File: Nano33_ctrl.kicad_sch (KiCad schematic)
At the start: 55 parts, among them J1 To Protec_Brd, J12 Conn_01x02, J15 To Display, J17 Conn_01x02, J18 To Protec_Brd encoder, J19 To P.A., J4 Power_In, J5 Conn_01x02, J6 Conn_01x02, U12 Arduino-NANO-33, U2 LM1117S-5.0, U3 LM1117S-3.3, U4 74HCT04, U5 TPIC6595, U6 TPIC6595, U7 TPIC6595, U8 24FC1025-I_SN, U9 24FC1025-I_SN

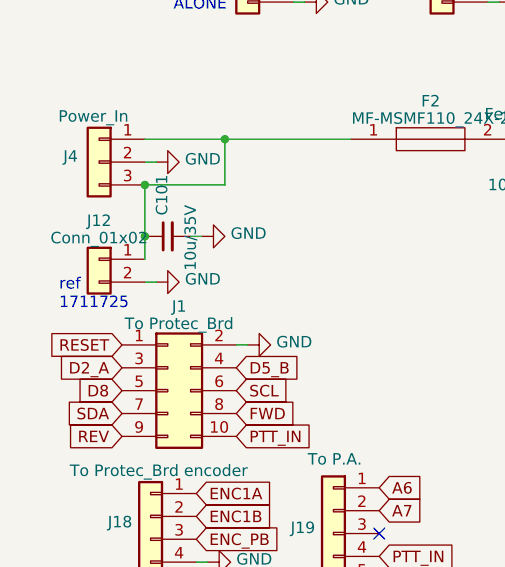
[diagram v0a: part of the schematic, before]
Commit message: more doc, silver mica bom
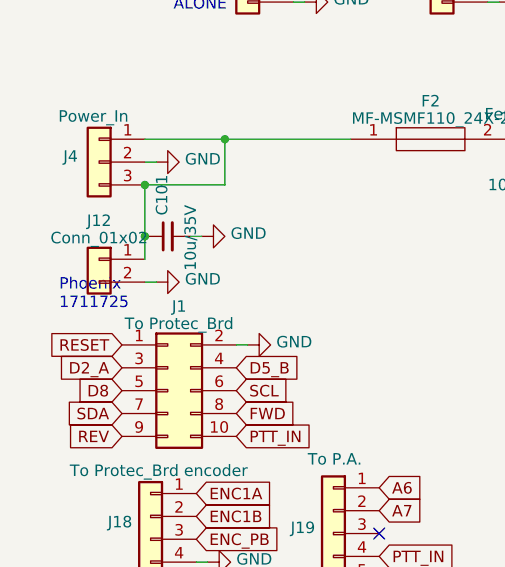
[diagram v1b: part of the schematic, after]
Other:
- note added: "Phoenix 1711725"
- note removed: "ref 1711725"
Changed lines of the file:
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@@
     (effects (font (size 1.27 1.27)) (justify left bottom))
   )
-  (text "ref\n1711725" (at 13.335 150.495 0)
+  (text "Phoenix\n1711725" (at 13.335 150.495 0)
     (effects (font (size 1.27 1.27)) (justify left bottom))
   )
